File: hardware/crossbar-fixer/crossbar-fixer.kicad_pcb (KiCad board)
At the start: 2 copper layers, 2 parts

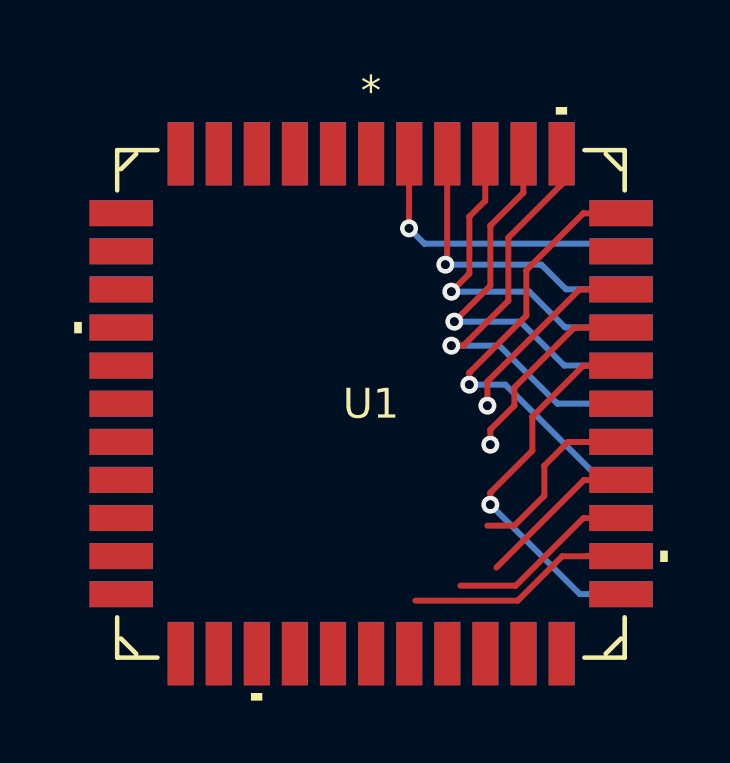
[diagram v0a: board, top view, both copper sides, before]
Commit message: I ate the fillet 'o fish
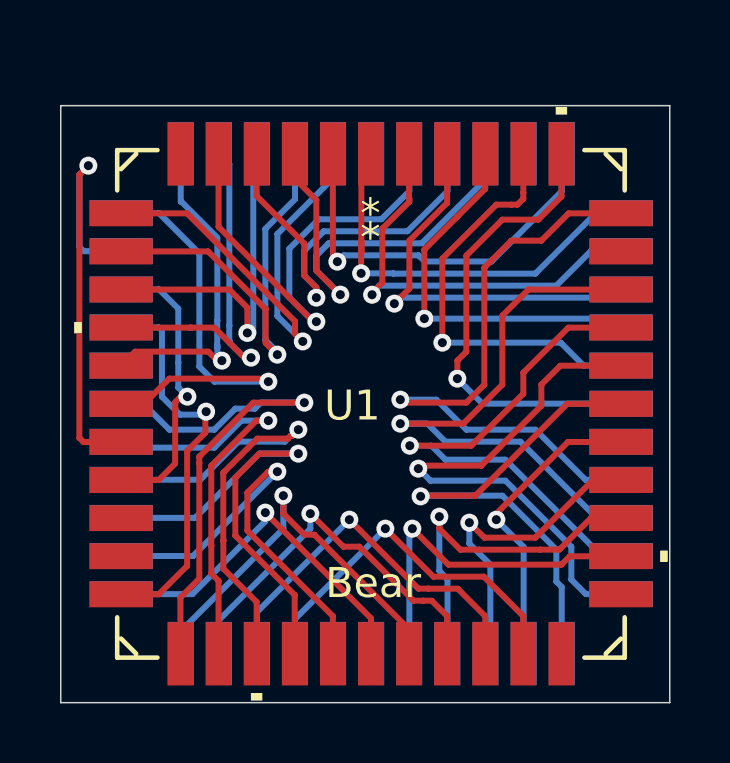
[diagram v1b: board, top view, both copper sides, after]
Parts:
- renumbered Fucked1 to U2
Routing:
- net Net-(U1-VSS): track 0.00 -> 17.9 mm, vias 0 -> 1
- net Net-(U1-X3): track 0.00 -> 16.8 mm, vias 0 -> 1
- net Net-(U1-STROBE): track 0.00 -> 16.2 mm, vias 0 -> 1
- net Net-(U1-Y5): track 0.00 -> 15.9 mm, vias 0 -> 1
- net Net-(U1-AX0): track 0.00 -> 15.9 mm, vias 0 -> 1
- net Net-(U1-X14): track 0.00 -> 15.4 mm, vias 0 -> 1
- net Net-(U1-X15): track 0.00 -> 15.0 mm, vias 0 -> 1
- net Net-(U1-X10): track 0.00 -> 14.9 mm, vias 0 -> 1
- net Net-(U1-X9): track 0.00 -> 14.7 mm, vias 0 -> 1
- net Net-(U1-RST): track 0.00 -> 14.5 mm, vias 0 -> 1
- net Net-(U1-Y6): track 0.00 -> 14.3 mm, vias 0 -> 1
- net Net-(U1-VEE): track 0.00 -> 14.2 mm, vias 0 -> 1
- net Net-(U1-AX3): track 0.00 -> 14.2 mm, vias 0 -> 1
- net Net-(U1-Y3): track 0.00 -> 14.0 mm, vias 0 -> 1
- net Net-(U1-AX1): track 0.00 -> 13.9 mm, vias 0 -> 1
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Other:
- board outline added: 20.3 x 19.9 mm
- board text added: "Bear"
- board text added: "Twink"
